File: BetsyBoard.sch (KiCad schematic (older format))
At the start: 40 parts, among them J1 USB_B_Micro, J2 Micro_SD_Card, P1 VDD, P2 VBUS, P3 CORTEX-JTAG, P4 Analog, P5 Digital, P6 BATT, P7 RTC, SW1 DIPSW, SW2 RST, U1 LP5907MFX, U2 USBLC6-2SC6, U3 APX823, U4 STM32L486Rx-LQFP64, X1 XTAL, Y1 Crystal

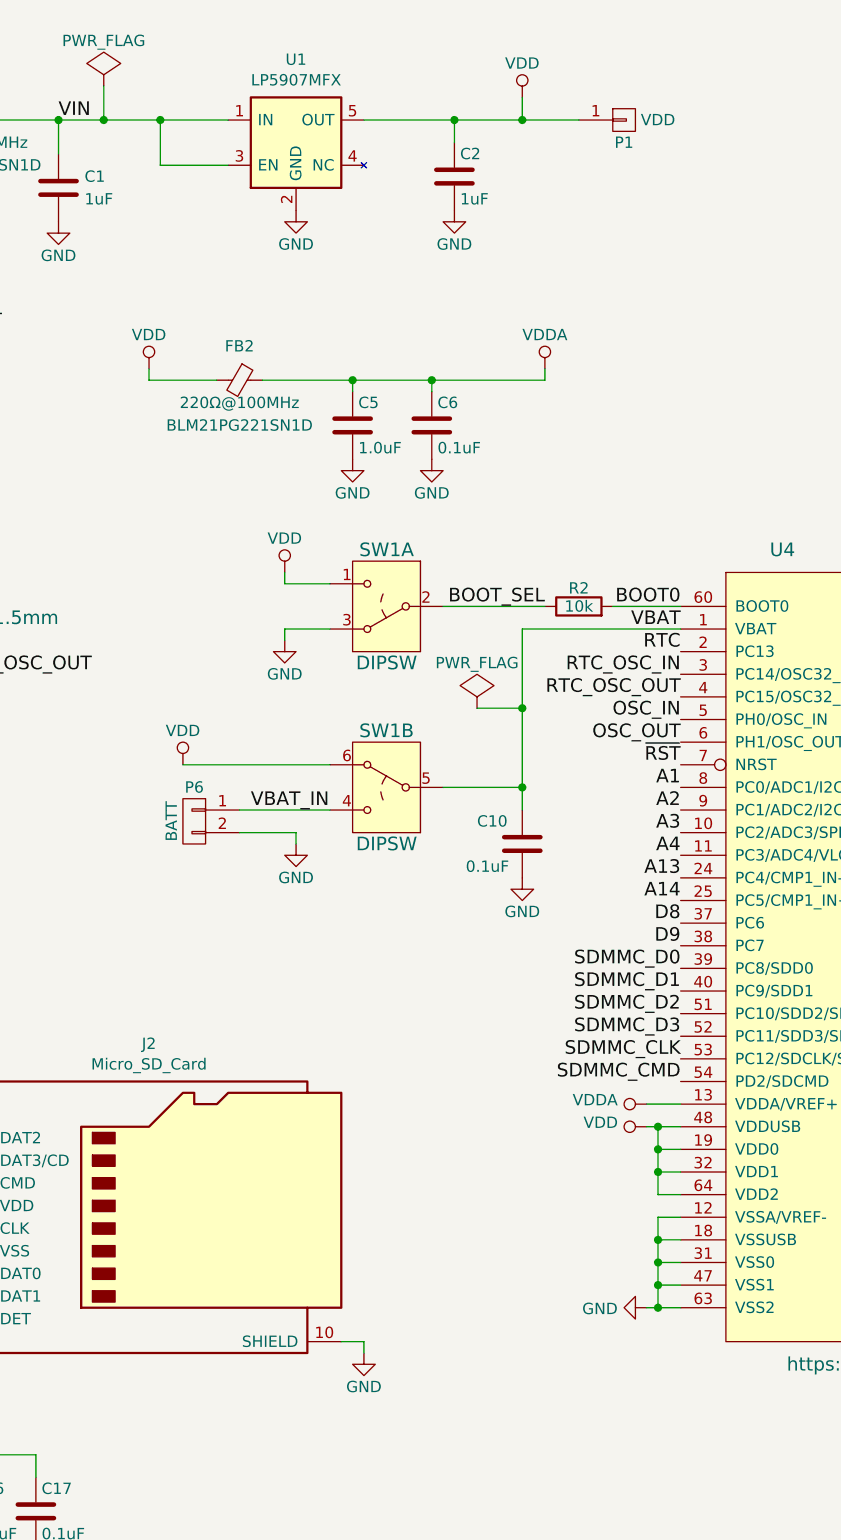
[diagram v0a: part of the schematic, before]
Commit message: More changes
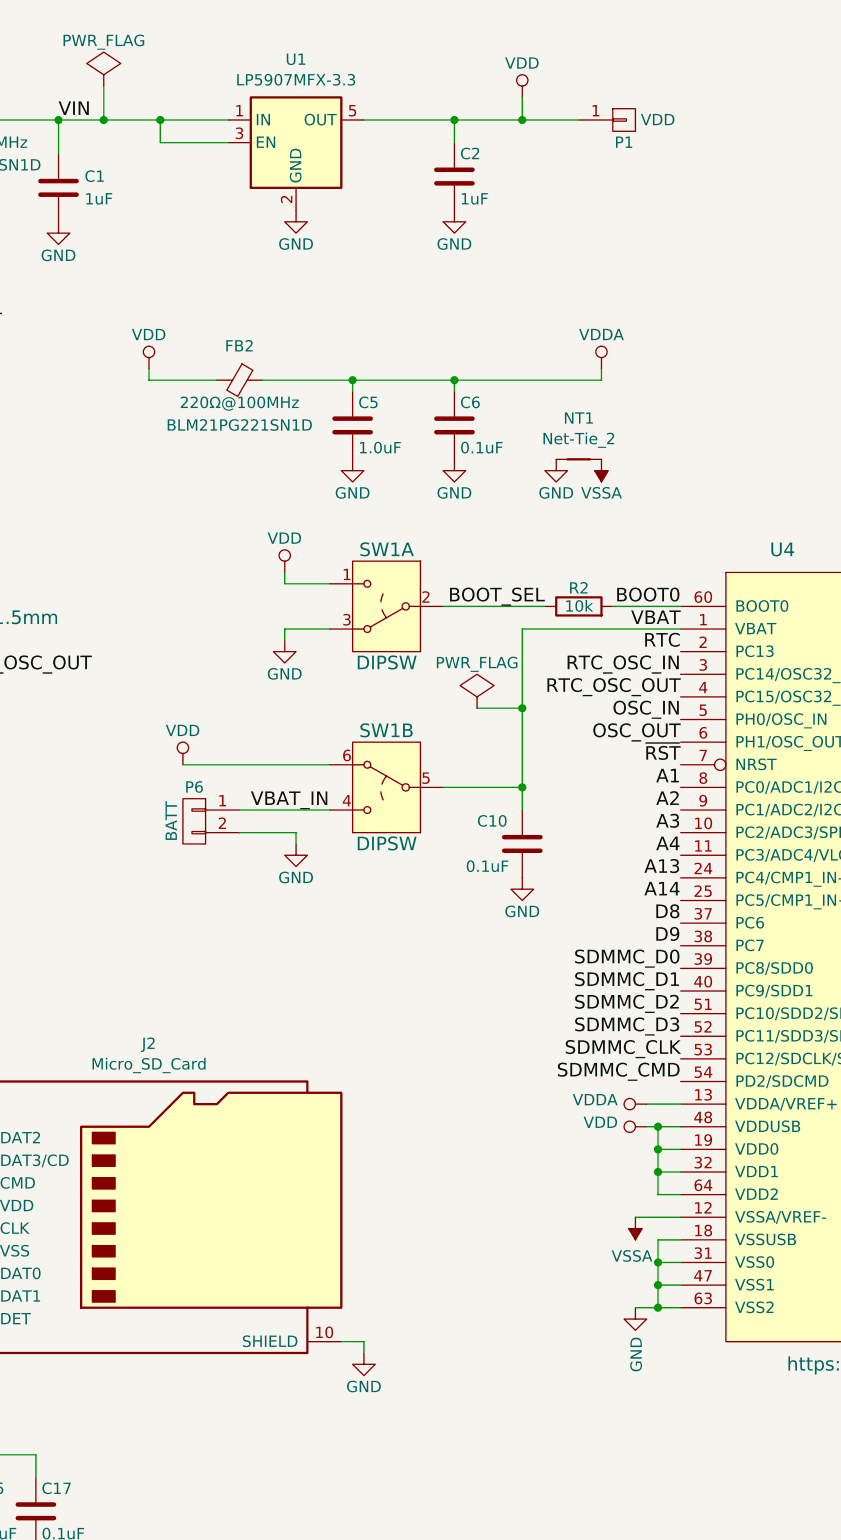
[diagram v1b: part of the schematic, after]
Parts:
- removed U1: LP5907MFX, Package_TO_SOT_SMD:SOT-23-5, symbol BetsyBoard-rescue:LP5907MFX
- added NT1: Net-Tie_2, NetTie:NetTie-2_SMD_Pad0.5mm, symbol Device:Net-Tie_2
- added U1: LP5907MFX-3.3, Package_TO_SOT_SMD:SOT-23-5, symbol Regulator_Linear:LP5907MFX-3.3
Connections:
- net GND: now also NT1.1, U1.2 (GND); no longer U4.12 (VSSA/VREF-)
- net VDD: now also U1.5 (OUT)
- net VIN: now also U1.1 (IN), U1.3 (EN)
- new net VSSA: NT1.2, U4.12 (VSSA/VREF-)
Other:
- moved on the sheet: C6
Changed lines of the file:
@@
 L BetsyBoard-rescue:C C6
 U 1 1 55FB1A93
-P 5100 2300
-F 0 "C6" H 5125 2400 50  0000 L CNN
-F 1 "0.1uF" H 5125 2200 50  0000 L CNN
-F 2 "Capacitor_SMD:C_0603_1608Metric" H 5138 2150 30  0001 C CNN
-F 3 "" H 5100 2300 60  0000 C CNN
-	1    5100 2300
+P 5200 2300
+F 0 "C6" H 5225 2400 50  0000 L CNN
+F 1 "0.1uF" H 5225 2200 50  0000 L CNN
+F 2 "Capacitor_SMD:C_0603_1608Metric" H 5238 2150 30  0001 C CNN
+F 3 "" H 5200 2300 60  0000 C CNN
+	1    5200 2300
 	1    0    0    -1
 $EndComp
@@
 $EndComp
 $Comp
-L BetsyBoard-rescue:GND #PWR010
-U 1 1 5629DE3D
-P 5100 2450
-F 0 "#PWR010" H 5100 2200 50  0001 C CNN
-F 1 "GND" H 5100 2300 50  0000 C CNN
-F 2 "" H 5100 2450 60  0000 C CNN
-F 3 "" H 5100 2450 60  0000 C CNN
-	1    5100 2450
-	1    0    0    -1
-$EndComp
-$Comp
 L BetsyBoard-rescue:VDD #PWR011
 U 1 1 5629E0D9
@@
 	1    0    0    -1
 $EndComp
-$Comp
-L BetsyBoard-rescue:LP5907MFX U1
-U 1 1 58FD570E
-P 4500 1050
-F 0 "U1" H 4500 1417 50  0000 C CNN
-F 1 "LP5907MFX" H 4500 1326 50  0000 C CNN
-F 2 "Package_TO_SOT_SMD:SOT-23-5" H 4500 1050 50  0001 C CNN
-F 3 "" H 4500 1050 50  0000 C CNN
-	1    4500 1050
-	1    0    0    -1
-$EndComp
 Text Label 3450 950  0    60   ~ 0
 VIN
@@
 	4750 2100 4750 2150
 Wire Wire Line
-	5100 2100 5100 2150
+	5200 2100 5200 2150
 Connection ~ 4750 2100
-Connection ~ 5100 2100
+Connection ~ 5200 2100
 Wire Wire Line
 	4150 2100 3850 2100
@@
 	5900 3100 6200 3100
 Wire Wire Line
-	3900 950  3900 1150
-Wire Wire Line
-	3900 1150 4200 1150
+	3900 950  3900 1050
+Wire Wire Line
+	3900 1050 4200 1050
 Connection ~ 3900 950
 Wire Wire Line
@@
 L BetsyBoard-rescue:VDDA #PWR039
 U 1 1 58FDF596
-P 5600 2050
-F 0 "#PWR039" H 5600 1900 50  0001 C CNN
-F 1 "VDDA" H 5600 2200 50  0000 C CNN
-F 2 "" H 5600 2050 50  0001 C CNN
-F 3 "" H 5600 2050 50  0001 C CNN
-	1    5600 2050
-	1    0    0    -1
-$EndComp
-Wire Wire Line
-	5600 2100 5600 2050
+P 5850 2050
+F 0 "#PWR039" H 5850 1900 50  0001 C CNN
+F 1 "VDDA" H 5850 2200 50  0000 C CNN
+F 2 "" H 5850 2050 50  0001 C CNN
+F 3 "" H 5850 2050 50  0001 C CNN
+	1    5850 2050
+	1    0    0    -1
+$EndComp
+Wire Wire Line
+	5850 2100 5850 2050
 $Comp
 L BetsyBoard-rescue:VDDA #PWR040
@@
 L BetsyBoard-rescue:GND #PWR042
 U 1 1 58FE0727
-P 6050 6200
-F 0 "#PWR042" H 6050 5950 50  0001 C CNN
-F 1 "GND" V 6055 6072 50  0000 R CNN
-F 2 "" H 6050 6200 50  0001 C CNN
-F 3 "" H 6050 6200 50  0001 C CNN
-	1    6050 6200
-	0    1    1    0
-$EndComp
-Wire Wire Line
-	6050 6200 6100 6200
-Wire Wire Line
-	6200 5800 6100 5800
-Wire Wire Line
-	6100 5800 6100 5900
+P 6000 6200
+F 0 "#PWR042" H 6000 5950 50  0001 C CNN
+F 1 "GND" V 6005 6072 50  0000 R CNN
+F 2 "" H 6000 6200 50  0001 C CNN
+F 3 "" H 6000 6200 50  0001 C CNN
+	1    6000 6200
+	1    0    0    -1
+$EndComp
+Wire Wire Line
+	6000 6200 6100 6200
 Connection ~ 6100 6200
 Wire Wire Line
 	6200 5900 6100 5900
-Connection ~ 6100 5900
 Wire Wire Line
 	6200 6000 6100 6000
@@
 	3450 950  3650 950
 Wire Wire Line
-	4750 2100 5100 2100
-Wire Wire Line
-	5100 2100 5600 2100
+	4750 2100 5200 2100
+Wire Wire Line
+	5200 2100 5850 2100
 Wire Wire Line
 	2250 3400 2400 3400
@@
 Wire Wire Line
 	5500 3900 5500 4000
+$Comp
+L Regulator_Linear:LP5907MFX-3.3 U1
+U 1 1 5F6ED042
+P 4500 1050
+F 0 "U1" H 4500 1417 50  0000 C CNN
+F 1 "LP5907MFX-3.3" H 4500 1326 50  0000 C CNN
+F 2 "Package_TO_SOT_SMD:SOT-23-5" H 4500 1400 50  0001 C CNN
+F 3 "http://www.ti.com/lit/ds/symlink/lp5907.pdf" H 4500 1550 50  0001 C CNN
+	1    4500 1050
+	1    0    0    -1
+$EndComp
+$Comp
+L power:VSSA #PWR0103
+U 1 1 5F7AACB0
+P 6000 5800
+F 0 "#PWR0103" H 6000 5650 50  0001 C CNN
+F 1 "VSSA" H 6015 5973 50  0000 C CNN
+F 2 "" H 6000 5800 50  0001 C CNN
+F 3 "" H 6000 5800 50  0001 C CNN
+	1    6000 5800
+	-1   0    0    1
+$EndComp
+Wire Wire Line
+	6000 5800 6200 5800
+$Comp
+L Device:Net-Tie_2 NT1
+U 1 1 5F7C24DA
+P 5750 2450
+F 0 "NT1" H 5750 2631 50  0000 C CNN
+F 1 "Net-Tie_2" H 5750 2540 50  0000 C CNN
+F 2 "NetTie:NetTie-2_SMD_Pad0.5mm" H 5750 2450 50  0001 C CNN
+F 3 "~" H 5750 2450 50  0001 C CNN
+	1    5750 2450
+	1    0    0    -1
+$EndComp
+$Comp
+L BetsyBoard-rescue:GND #PWR0104
+U 1 1 5F7D17B7
+P 5650 2450
+F 0 "#PWR0104" H 5650 2200 50  0001 C CNN
+F 1 "GND" H 5650 2300 50  0000 C CNN
+F 2 "" H 5650 2450 60  0000 C CNN
+F 3 "" H 5650 2450 60  0000 C CNN
+	1    5650 2450
+	1    0    0    -1
+$EndComp
+$Comp
+L power:VSSA #PWR0105
+U 1 1 5F7D22B3
+P 5850 2450
+F 0 "#PWR0105" H 5850 2300 50  0001 C CNN
+F 1 "VSSA" H 5850 2600 50  0000 C CNN
+F 2 "" H 5850 2450 50  0001 C CNN
+F 3 "" H 5850 2450 50  0001 C CNN
+	1    5850 2450
+	-1   0    0    1
+$EndComp
+$Comp
+L BetsyBoard-rescue:GND #PWR?
+U 1 1 5F817E0A
+P 5200 2450
+F 0 "#PWR?" H 5200 2200 50  0001 C CNN
+F 1 "GND" H 5200 2300 50  0000 C CNN
+F 2 "" H 5200 2450 60  0000 C CNN
+F 3 "" H 5200 2450 60  0000 C CNN
+	1    5200 2450
+	1    0    0    -1
+$EndComp
 $EndSCHEMATC

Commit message: Fix rescued symbols
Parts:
- C1, C10, C11, C12, C13, C14, C15, C16, C17, C2, C3, C5, C6, C7: symbol BetsyBoard-rescue:C -> Device:C
- C8, C9: symbol BetsyBoard-rescue:C_Small -> Device:C_Small
- D1, D2: symbol BetsyBoard-rescue:LED-RESCUE-BetsyBoard -> Device:LED
- P1, P2: symbol BetsyBoard-rescue:CONN_01X01 -> Connector:Conn_01x01_Male
- P3: symbol BetsyBoard-rescue:CONN_02X05 -> Connector_Generic:Conn_02x05_Odd_Even
- P4, P5: symbol BetsyBoard-rescue:CONN_01X16 -> Connector_Generic:Conn_01x16
- P6: symbol BetsyBoard-rescue:CONN_01X02 -> Connector_Generic:Conn_01x02
- P7: symbol BetsyBoard-rescue:CONN_01X01 -> Connector_Generic:Conn_01x01
- R2, R3, R4: symbol BetsyBoard-rescue:R -> Device:R
- SW2: symbol BetsyBoard-rescue:SW_PUSH_NO -> @Engstad:SW_PUSH_NO
- U3: symbol BetsyBoard-rescue:APX823 -> @Engstad:APX823
- Y1: symbol BetsyBoard-rescue:Crystal -> Device:Crystal
